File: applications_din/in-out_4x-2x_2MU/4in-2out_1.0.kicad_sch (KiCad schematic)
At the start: 63 parts, among them IC1 ULN2803, J1 Con_CTRL, J2 Con_IO, J3 Con_230V, J4 Con_EIB_WAGO_243-211, J5 Con_230V, K1 HFE20-1/24-1HSD-L2, K2 HFE20-1/24-1HSD-L2, U1 74HC595, U2 74HC165, X9 W237-102

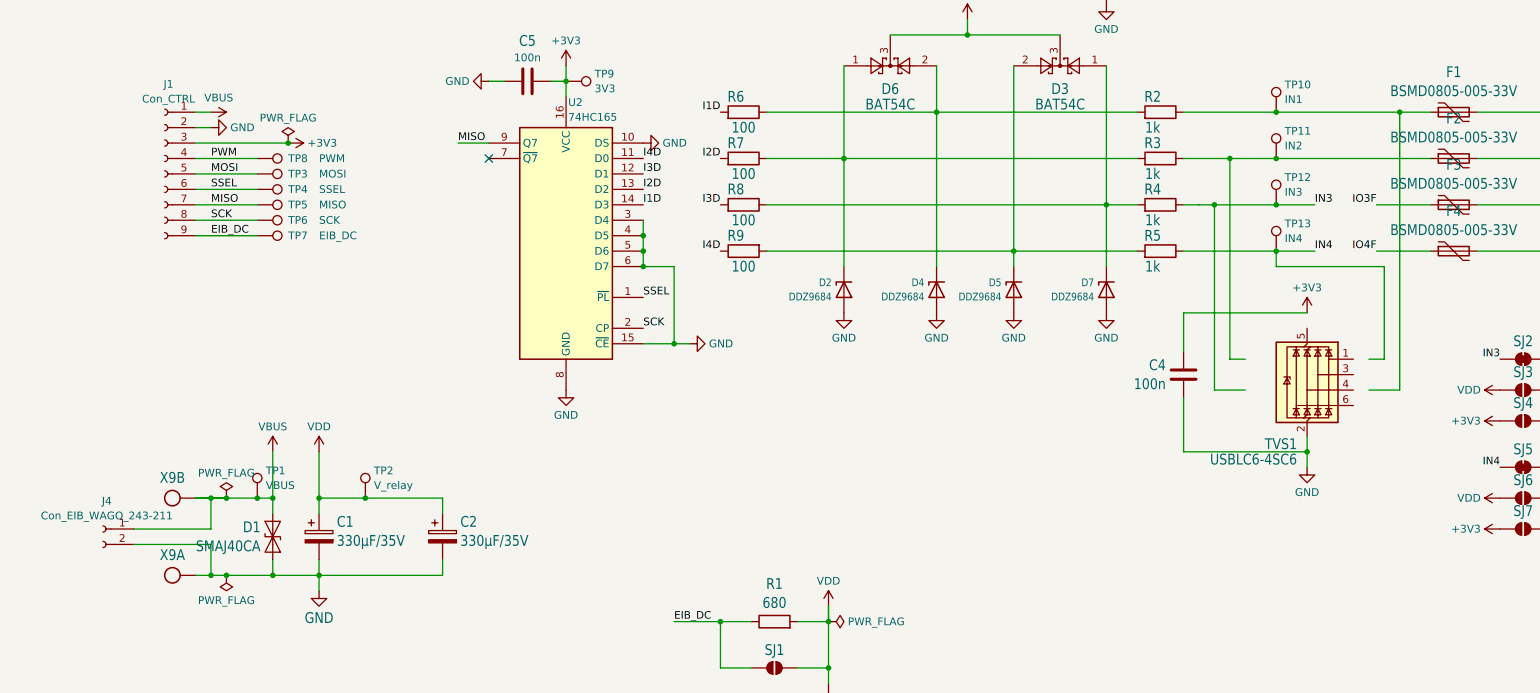
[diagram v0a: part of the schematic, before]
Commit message: update in-out_4x-2x_2MU - final for now
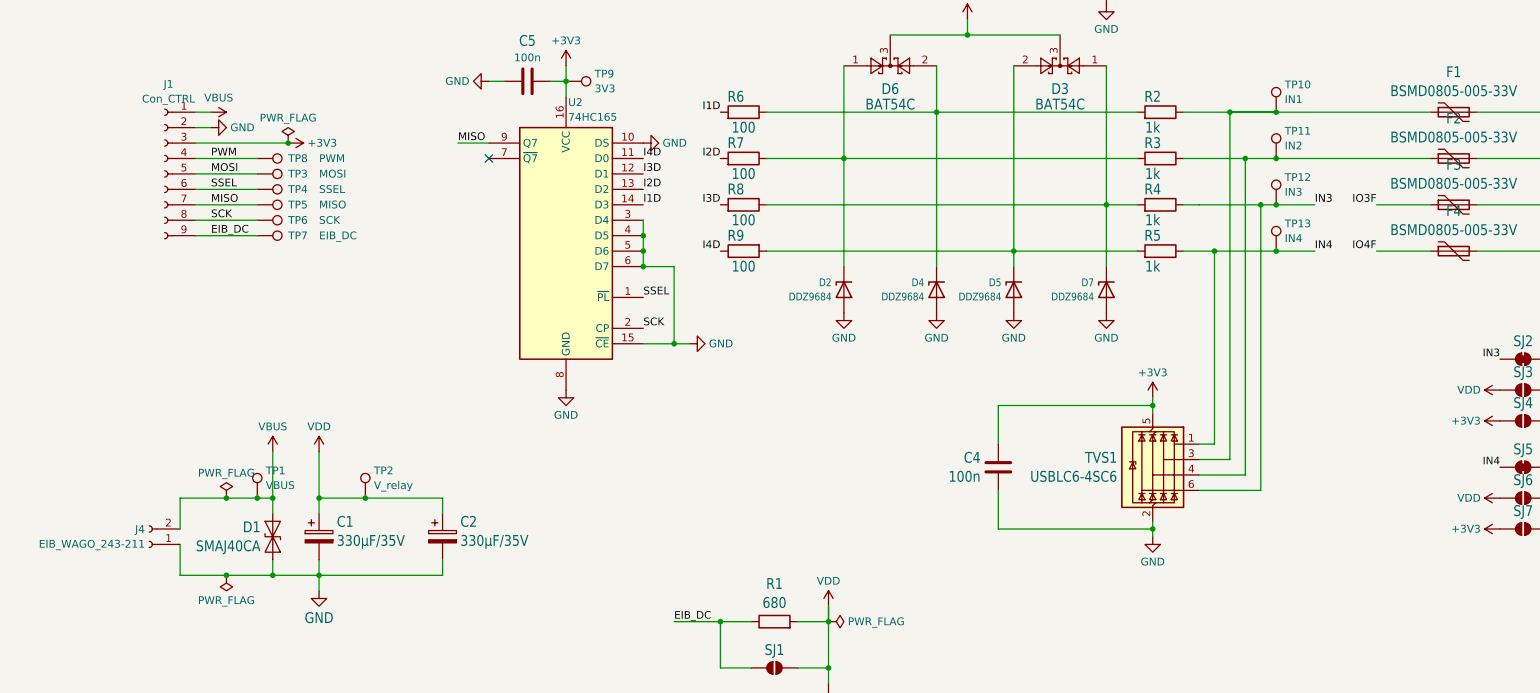
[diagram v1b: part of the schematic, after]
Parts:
- removed X9: W237-102, selfbus:W237-102, symbol selfbus:W237-102
- J4: value Con_EIB_WAGO_243-211 -> EIB_WAGO_243-211; footprint (none) -> selfbus:W243-211_1x02_P5.75
- K1, K2: footprint selfbus:HFE20-1-L2 -> selfbus:HFE20-GENERIC-COMBO
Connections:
- net +3V3: now also TVS1.5 (VBUS)
- net GND: now also J4.1 (Pin_1); no longer J4.2 (Pin_2)
- net IN3: now also TVS1.6 (I/O4)
- net IN4: now also TVS1.1 (I/O1)
- net VBUS: now also J4.2 (Pin_2); no longer J4.1 (Pin_1)
- net at F2.1, R3.1, TP11.1: now also TVS1.4 (I/O3)
- net at F1.1, R2.1, TP10.1: now also TVS1.3 (I/O2)
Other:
- moved on the sheet: C4, J4, TVS1
